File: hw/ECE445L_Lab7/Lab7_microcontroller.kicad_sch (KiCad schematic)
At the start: 17 parts, among them U4 M0G3507QDGS32RQ1, U6 M0G3507QDGS32RQ1, Y1 16MHz, Y2 16MHz

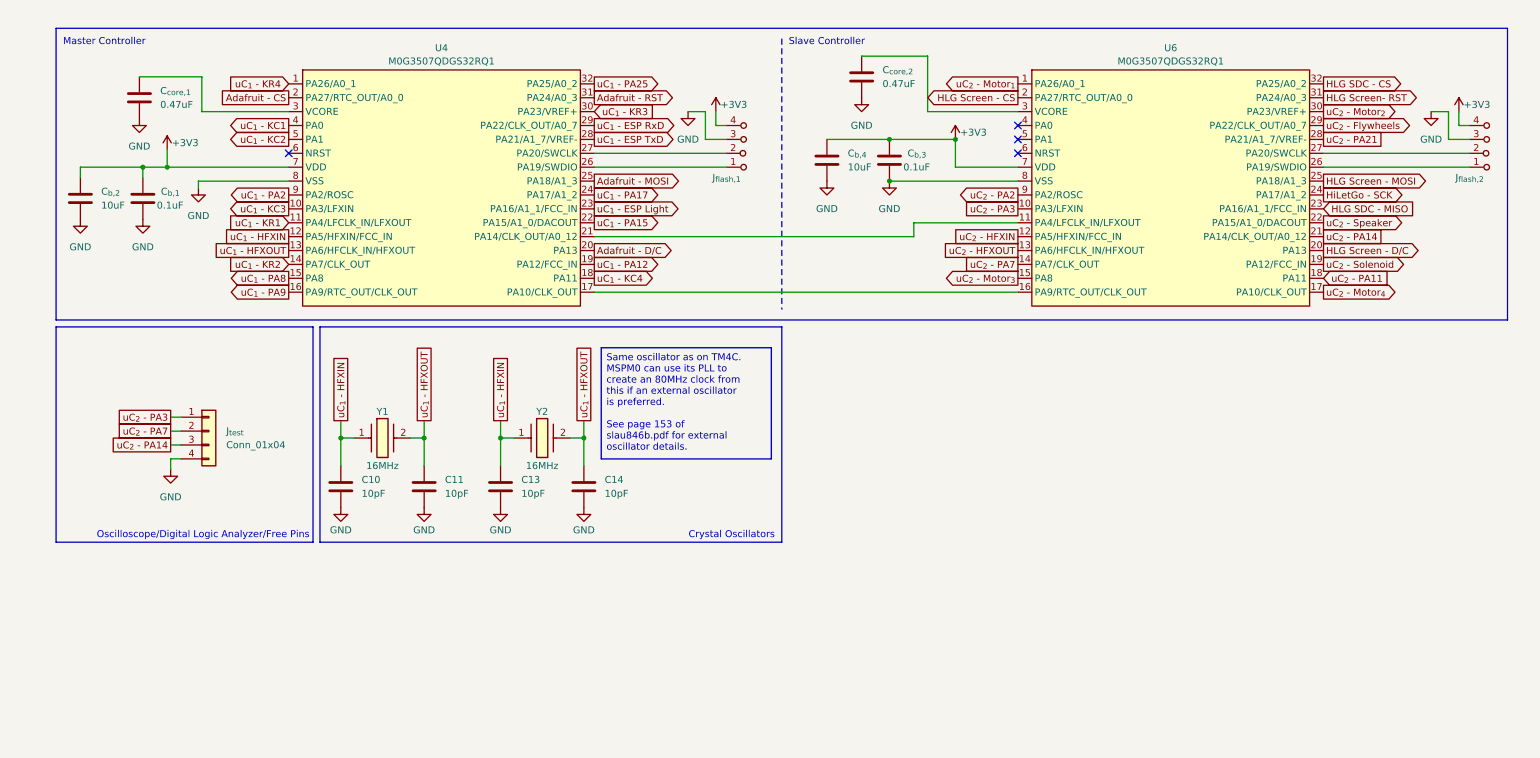
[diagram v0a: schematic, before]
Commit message: almost finished with schem
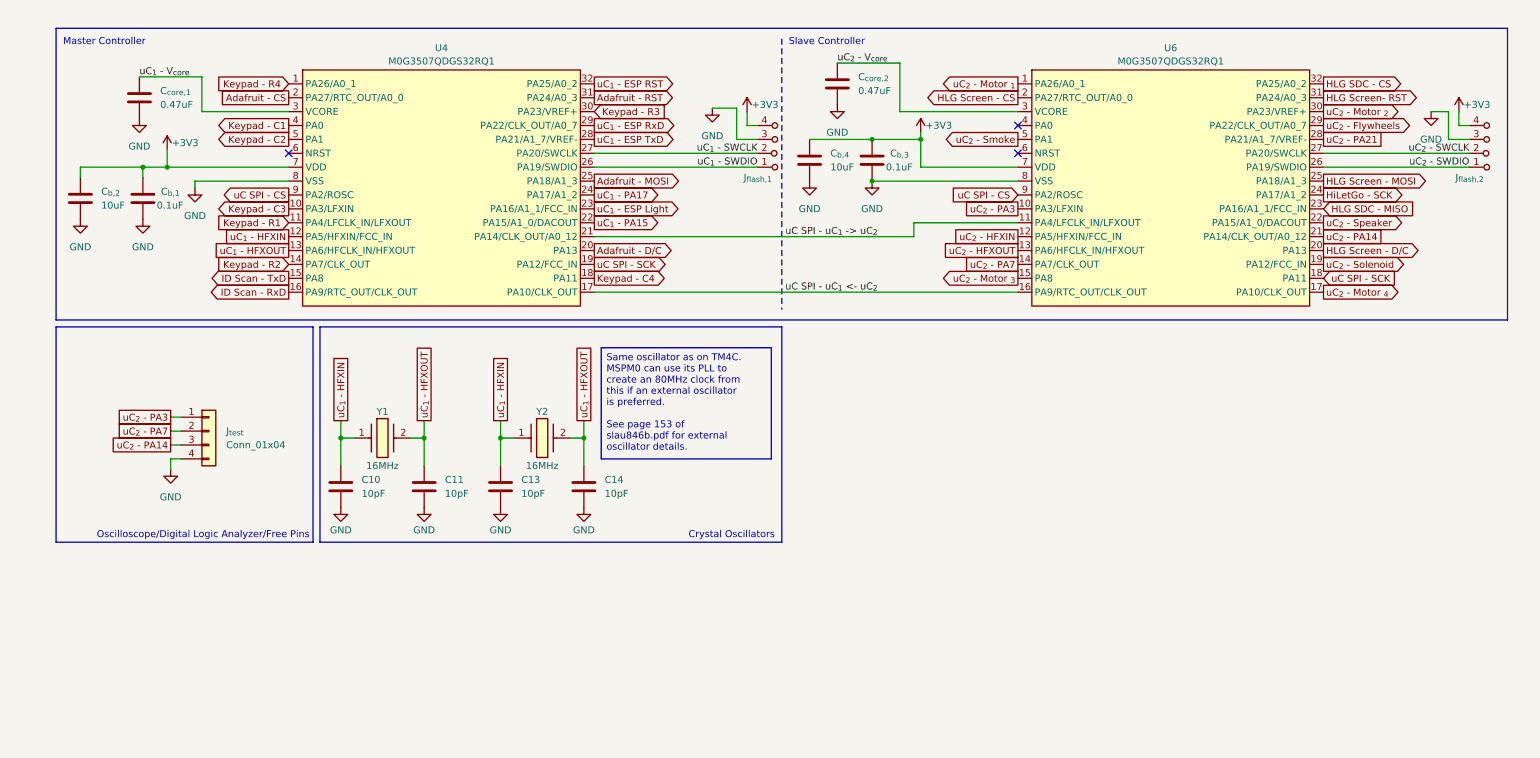
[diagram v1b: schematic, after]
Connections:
- net uC_{2} - PA11 is gone; now on net uC SPI - SCK: U6.18 (PA11)
- net uC_{2} - PA2 is gone; now on net uC SPI - CS: U6.9 (PA2/ROSC)
- net uC_{1} - SWDIO: now reaches J_{flash,1}.1 (A), U4.26 (PA19/SWDIO)
- net uC_{1} - SWCLK: now reaches J_{flash,1}.2 (B), U4.27 (PA20/SWCLK)
- net uC_{1} - V_{core}: now reaches C_{core,1}.1, U4.3 (VCORE)
- net uC_{2} - SWDIO: now reaches J_{flash,2}.1 (A), U6.26 (PA19/SWDIO)
- net uC_{2} - SWCLK: now reaches J_{flash,2}.2 (B), U6.27 (PA20/SWCLK)
- net uC_{2} - V_{core}: now reaches C_{core,2}.1, U6.3 (VCORE)
- net uC SPI - uC_{1} -> uC_{2}: now reaches U4.21 (PA14/CLK_OUT/A0_12), U6.11 (PA4/LFCLK_IN/LFXOUT)
- net uC SPI - uC_{1} <- uC_{2}: now reaches U4.17 (PA10/CLK_OUT), U6.16 (PA9/RTC_OUT/CLK_OUT)
- net uC_{2} - Smoke: now reaches U6.5 (PA1)
- net uC_{1} - KC1 renamed Keypad - C1
- net uC_{1} - KC2 renamed Keypad - C2
- net uC_{1} - KC3 renamed Keypad - C3
- net uC_{1} - KC4 renamed Keypad - C4
- net uC_{1} - KR1 renamed Keypad - R1
- net uC_{1} - KR2 renamed Keypad - R2
- net uC_{1} - KR3 renamed Keypad - R3
- net uC_{1} - KR4 renamed Keypad - R4
- net uC_{1} - PA12 renamed uC SPI - SCK
- net uC_{1} - PA2 renamed uC SPI - CS
- net uC_{1} - PA25 renamed uC_{1} - ESP RST
- net uC_{1} - PA8 renamed ID Scan - TxD
- net uC_{1} - PA9 renamed ID Scan - RxD
- net uC_{2} - Motor_{1} renamed uC_{2} - Motor _{1}
- net uC_{2} - Motor_{2} renamed uC_{2} - Motor _{2}
- net uC_{2} - Motor_{3} renamed uC_{2} - Motor _{3}
- net uC_{2} - Motor_{4} renamed uC_{2} - Motor _{4}
- no-connect marks 4 -> 3
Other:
- moved on the sheet: C_{b,3}, C_{b,4}, C_{core,2}, J_{flash,1}

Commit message: finished prelim schem
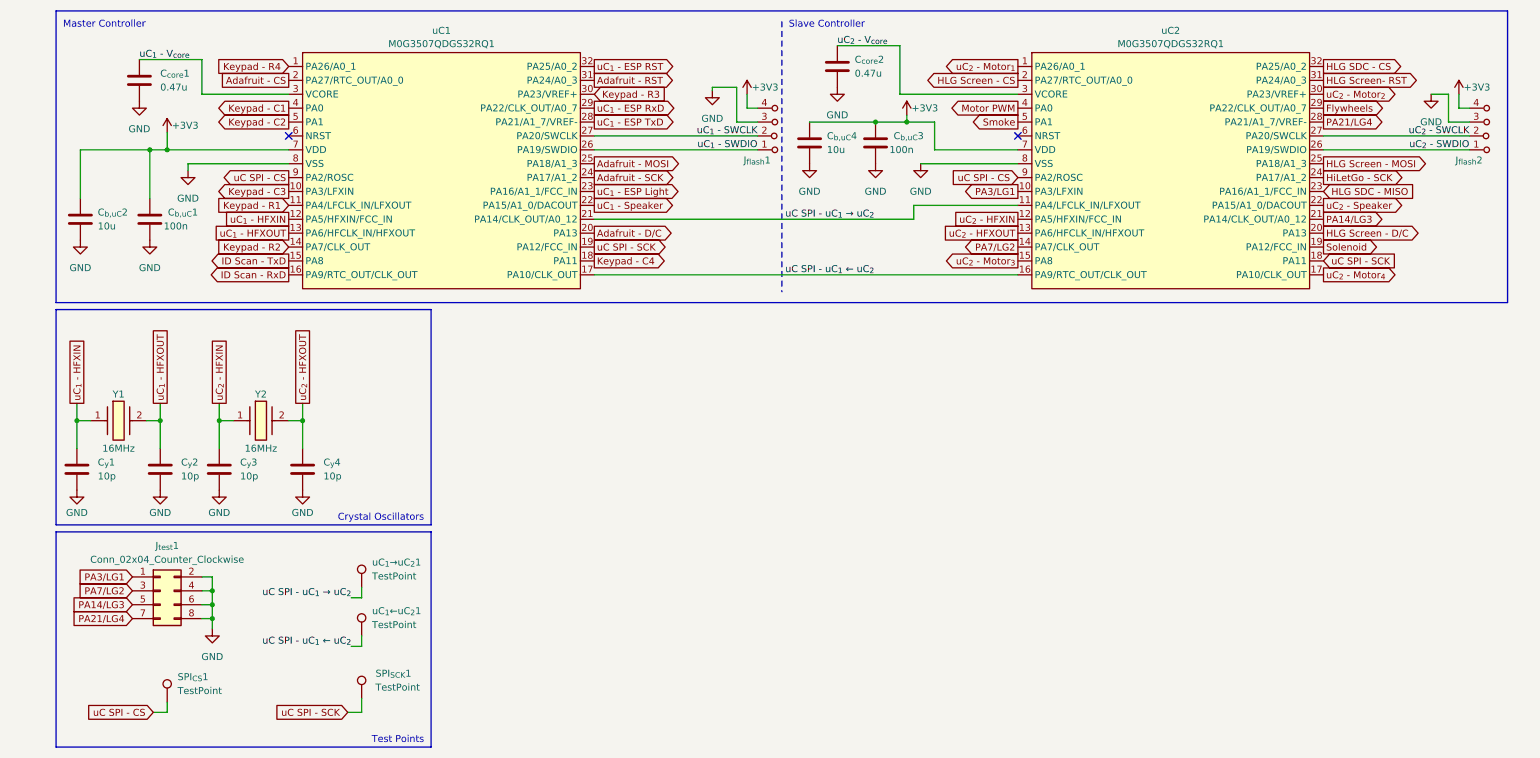
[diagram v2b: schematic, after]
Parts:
- removed J_{test}: Conn_01x04, Connector_PinHeader_2.54mm:PinHeader_1x04_P2.54mm_Vertical, symbol Connector_Generic:Conn_01x04
- added J_{test}1: Conn_02x04_Counter_Clockwise, Connector_PinSocket_2.54mm:PinSocket_2x04_P2.54mm_Vertical, symbol Connector_Generic:Conn_02x04_Odd_Even
- added SPI_{CS}1, SPI_{SCK}1, uC_{1}←uC_{2}1, uC_{1}→uC_{2}1: TestPoint, TestPoint:TestPoint_Keystone_5010-5014_Multipurpose, symbol Connector:TestPoint
- C_{b,uC}1: renamed from C_{b,1}; value 0.1uF -> 100n; footprint ECE445L:C_Radial_100mil -> Capacitor_SMD:C_0603_1608Metric_Pad1.08x0.95mm_HandSolder; Distributor (none) -> Mouser; Manufacturer (none) -> Walsin; Manufacturer_Part_Number (none) -> 0603B104J160CT; Mouser Part Number (none) -> 791-0603B104J160CT
- C_{b,uC}2: renamed from C_{b,2}; value 10uF -> 10u; footprint ECE445L:C_Radial_100mil -> Capacitor_SMD:C_0603_1608Metric_Pad1.08x0.95mm_HandSolder; Distributor (none) -> Mouser; Manufacturer (none) -> TDK; Manufacturer_Part_Number (none) -> C1608X7T1A106M080AC; Mouser Part Number (none) -> 810-C1608X7T1A106M08
- C_{b,uC}3: renamed from C_{b,3}; value 0.1uF -> 100n; footprint ECE445L:C_Radial_100mil -> Capacitor_SMD:C_0603_1608Metric_Pad1.08x0.95mm_HandSolder; Distributor (none) -> Mouser; Manufacturer (none) -> Walsin; Manufacturer_Part_Number (none) -> 0603B104J160CT; Mouser Part Number (none) -> 791-0603B104J160CT
- C_{b,uC}4: renamed from C_{b,4}; value 10uF -> 10u; footprint ECE445L:C_Radial_100mil -> Capacitor_SMD:C_0603_1608Metric_Pad1.08x0.95mm_HandSolder; Distributor (none) -> Mouser; Manufacturer (none) -> TDK; Manufacturer_Part_Number (none) -> C1608X7T1A106M080AC; Mouser Part Number (none) -> 810-C1608X7T1A106M08
- C_{core}1: renamed from C_{core,1}; value 0.47uF -> 0.47u; footprint Capacitor_SMD:C_0201_0603Metric_Pad0.64x0.40mm_HandSolder -> Capacitor_SMD:C_0603_1608Metric_Pad1.08x0.95mm_HandSolder; Distributor (none) -> Mouser; Manufacturer (none) -> Walsin; Manufacturer_Part_Number (none) -> 0603B474K6R3CT; Mouser Part Number (none) -> 791-0603B474K6R3CT
- C_{core}2: renamed from C_{core,2}; value 0.47uF -> 0.47u; footprint Capacitor_SMD:C_0201_0603Metric_Pad0.64x0.40mm_HandSolder -> Capacitor_SMD:C_0603_1608Metric_Pad1.08x0.95mm_HandSolder; Distributor (none) -> Mouser; Manufacturer (none) -> Walsin; Manufacturer_Part_Number (none) -> 0603B474K6R3CT; Mouser Part Number (none) -> 791-0603B474K6R3CT
- C_{y}1: renamed from C10; value 10pF -> 10p; footprint Capacitor_SMD:C_0201_0603Metric_Pad0.64x0.40mm_HandSolder -> Capacitor_SMD:C_0603_1608Metric_Pad1.08x0.95mm_HandSolder; Distributor (none) -> Mouser; Manufacturer (none) -> Walsin; Manufacturer_Part_Number (none) -> 0603N100F101CT; Mouser Part Number (none) -> 791-0603N100F101CT
- C_{y}2: renamed from C11; value 10pF -> 10p; footprint Capacitor_SMD:C_0201_0603Metric_Pad0.64x0.40mm_HandSolder -> Capacitor_SMD:C_0603_1608Metric_Pad1.08x0.95mm_HandSolder; Distributor (none) -> Mouser; Manufacturer (none) -> Walsin; Manufacturer_Part_Number (none) -> 0603N100F101CT; Mouser Part Number (none) -> 791-0603N100F101CT
- C_{y}3: renamed from C13; value 10pF -> 10p; footprint Capacitor_SMD:C_0201_0603Metric_Pad0.64x0.40mm_HandSolder -> Capacitor_SMD:C_0603_1608Metric_Pad1.08x0.95mm_HandSolder; Distributor (none) -> Mouser; Manufacturer (none) -> Walsin; Manufacturer_Part_Number (none) -> 0603N100F101CT; Mouser Part Number (none) -> 791-0603N100F101CT
- C_{y}4: renamed from C14; value 10pF -> 10p; footprint Capacitor_SMD:C_0201_0603Metric_Pad0.64x0.40mm_HandSolder -> Capacitor_SMD:C_0603_1608Metric_Pad1.08x0.95mm_HandSolder; Distributor (none) -> Mouser; Manufacturer (none) -> Walsin; Manufacturer_Part_Number (none) -> 0603N100F101CT; Mouser Part Number (none) -> 791-0603N100F101CT
- Y1, Y2: Manufacturer (none) -> ABRACON
- renumbered J_{flash,1} to J_{flash}1, J_{flash,2} to J_{flash}2, U4 to uC1, U6 to uC2
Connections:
- net GND: now also J_{test}1.2 (Pin_2), J_{test}1.4 (Pin_4), J_{test}1.6 (Pin_6), J_{test}1.8 (Pin_8)
- net uC SPI - CS: now also SPI_{CS}1.1
- net uC SPI - SCK: now also SPI_{SCK}1.1
- net uC_{1} - HFXIN: no longer C_{y}3.1, Y2.1
- net uC_{1} - HFXOUT: no longer C_{y}4.1, Y2.2
- net uC_{2} - HFXIN: now also C_{y}3.1, Y2.1
- net uC_{2} - HFXOUT: now also C_{y}4.1, Y2.2
- net Motor PWM: now reaches uC2.4 (PA0)
- net uC SPI - uC_{1} -> uC_{2} renamed uC SPI - uC_{1} → uC_{2}
- net uC SPI - uC_{1} → uC_{2}: now also uC_{1}→uC_{2}1.1
- net uC SPI - uC_{1} <- uC_{2} renamed uC SPI - uC_{1} ← uC_{2}
- net uC SPI - uC_{1} ← uC_{2}: now also uC_{1}←uC_{2}1.1
- net uC_{1} - PA15 renamed uC_{1} - Speaker
- net uC_{1} - PA17 renamed Adafruit - SCK
- net uC_{2} - Flywheels renamed Flywheels
- net uC_{2} - Motor _{1} renamed uC_{2} - Motor_{1}
- net uC_{2} - Motor _{2} renamed uC_{2} - Motor_{2}
- net uC_{2} - Motor _{3} renamed uC_{2} - Motor_{3}
- net uC_{2} - Motor _{4} renamed uC_{2} - Motor_{4}
- net uC_{2} - PA14 renamed PA14/LG3
- net PA14/LG3: now also J_{test}1.5 (Pin_5)
- net uC_{2} - PA21 renamed PA21/LG4
- net PA21/LG4: now also J_{test}1.7 (Pin_7)
- net uC_{2} - PA3 renamed PA3/LG1
- net PA3/LG1: now also J_{test}1.1 (Pin_1)
- net uC_{2} - PA7 renamed PA7/LG2
- net PA7/LG2: now also J_{test}1.3 (Pin_3)
- net uC_{2} - Smoke renamed Smoke
- net uC_{2} - Solenoid renamed Solenoid
- no-connect marks 3 -> 2
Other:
- note added: "Test Points"
- note removed: "Oscilloscope/Digital Logic Analyzer/Free Pins"
- moved on the sheet: C_{b,uC}1, C_{b,uC}2, C_{b,uC}3, C_{b,uC}4, C_{core}1, C_{core}2, C_{y}1, C_{y}2, C_{y}3, C_{y}4, J_{flash}1, J_{flash}2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
